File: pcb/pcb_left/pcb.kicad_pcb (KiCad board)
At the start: 2 copper layers, 154 x 108.3 mm, 62 parts, among them J1 OLED_128x32, U1 Nice_Nano_V2

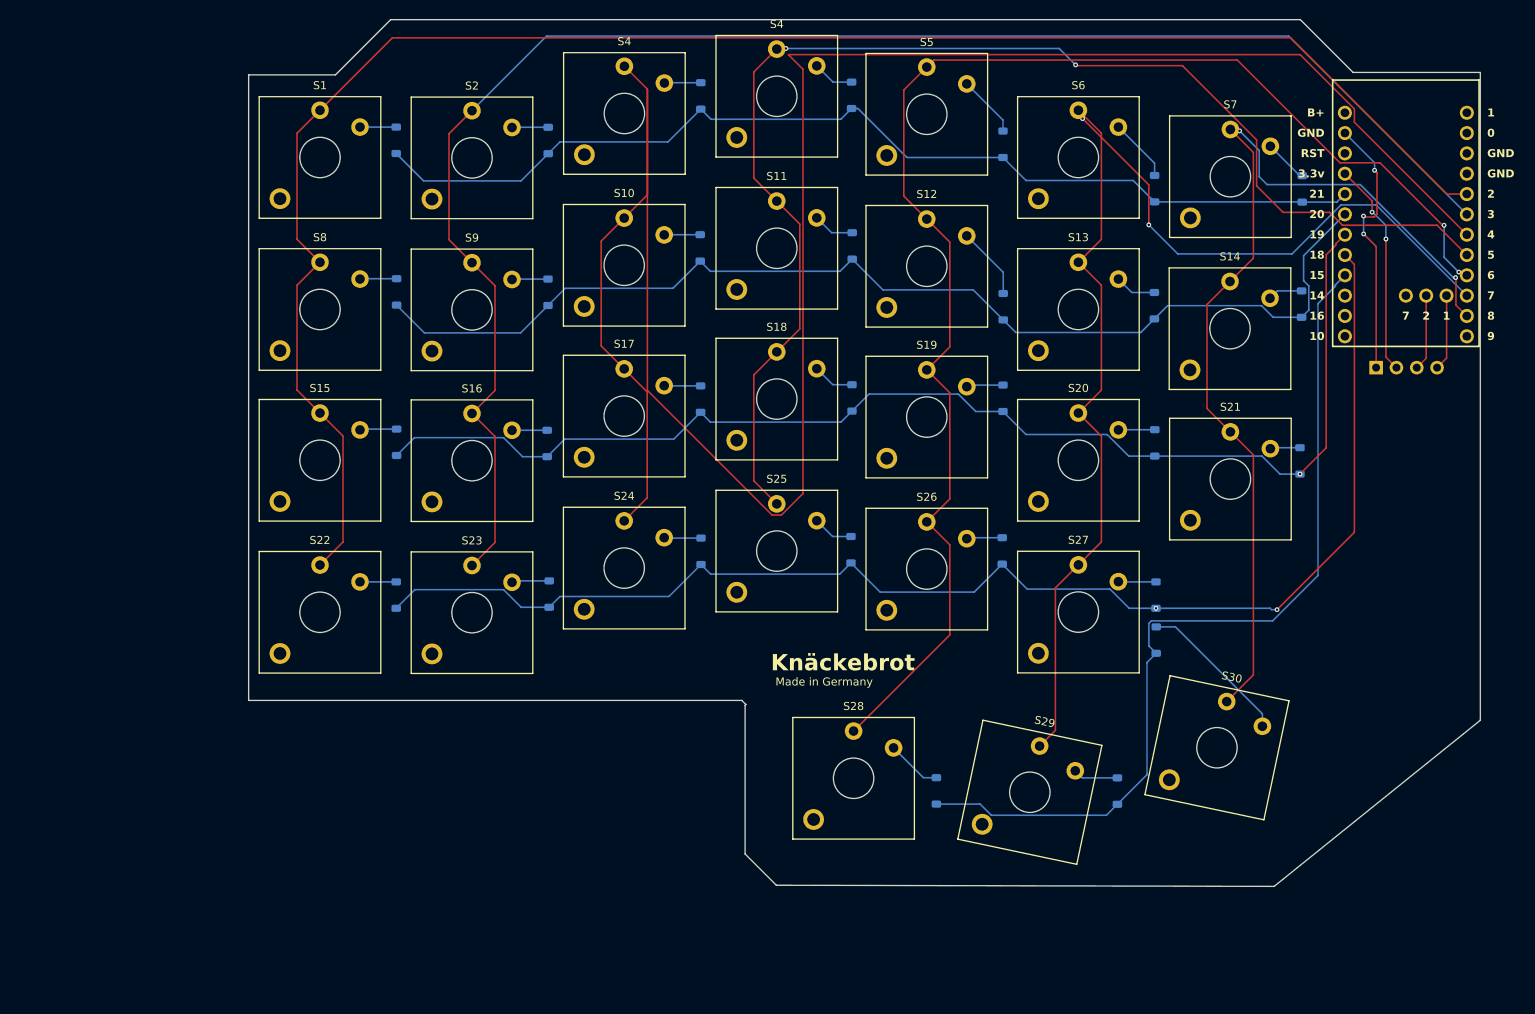
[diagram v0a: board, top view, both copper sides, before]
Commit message: Upadate v1.00
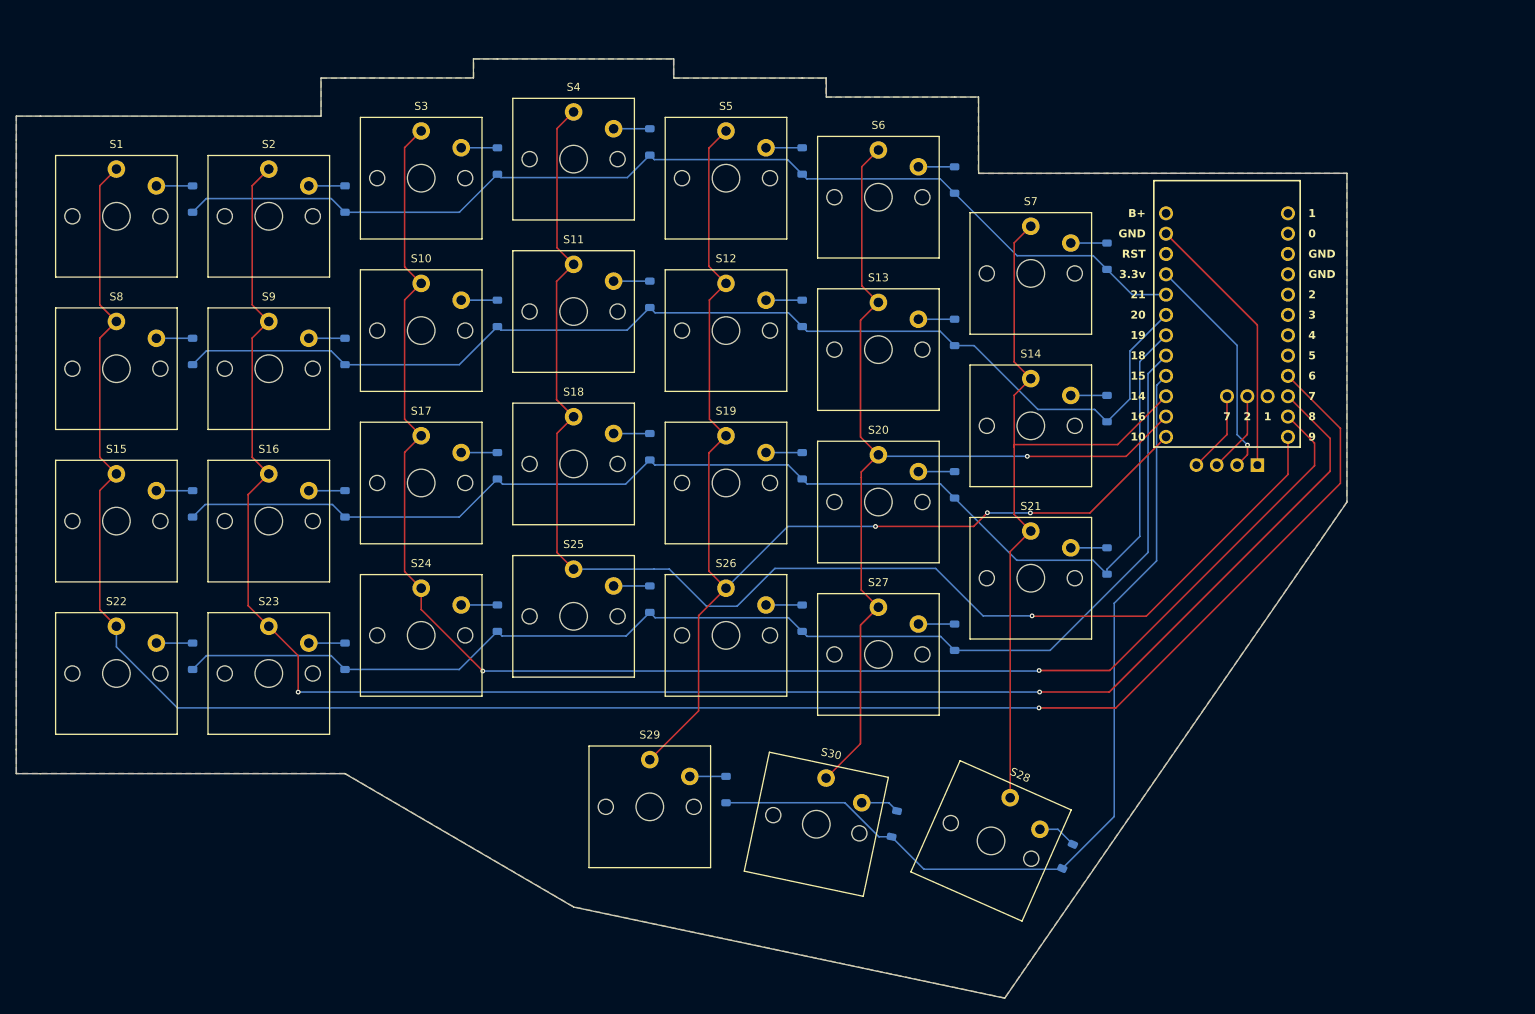
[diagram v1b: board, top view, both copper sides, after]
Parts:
- removed the S4 at (107.8, 47.8)
- removed the S4 at (126.8, 45.6)
- added S3: Keyswitch, ScottoKeebs_Choc:Choc_V1, F.Cu at (82.4, 55.9)
- added S4: Keyswitch, ScottoKeebs_Choc:Choc_V1, F.Cu at (101.4, 53.5)
- D1, D10, D11, D12, D13, D14, D15, D16, D17, D18, D19, D2, D20, D21, D22, D23, D24, D25, D26, D27, D28, D29, D3, D30, D4, D5, D6, D7, D8, D9: footprint Diode_SMD:D_SOD-123 -> ScottoKeebs_Components:Diode_SOD-123
- S1, S10, S11, S12, S13, S14, S15, S16, S17, S18, S19, S2, S20, S21, S22, S23, S24, S25, S26, S27, S28, S29, S30, S5, S6, S7, S8, S9: footprint ScottoKeebs_Choc:Choc_V2 -> ScottoKeebs_Choc:Choc_V1
- moved S30 51.0 mm to (131.8, 136.6)
- moved D29 48.9 mm to (120.5, 132.3)
- moved S29 47.5 mm to (111.0, 134.5), turned to 0 degrees
- moved D30 40.0 mm to (141.5, 136.6), turned to 78.06 degrees
- moved J1 37.7 mm to (177.1, 93.4), turned to 90 degrees
- moved S21 27.9 mm to (158.6, 105.9)
- moved S7 27.7 mm to (158.6, 67.8)
- moved S14 27.7 mm to (158.6, 86.8)
- moved D14 27.6 mm to (168.1, 84.7)
- moved D21 27.2 mm to (168.1, 103.7)
- moved D24 26.8 mm to (91.9, 110.9)
- moved D17 26.7 mm to (91.9, 91.8)
- moved S24 26.7 mm to (82.4, 113.0)
- moved S17 26.7 mm to (82.4, 94.0)
- moved D3 26.7 mm to (91.9, 53.7)
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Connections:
- net Row_0_L renamed row 0
- net Row_1_L renamed row 1
- net Row_2_L renamed row 2
- net Row_3_L renamed row 3
- net Row_4_L renamed row 4
- S1 pad 1: Col_0_L -> column 0
- S10 pad 1: Col_2_L -> column 2
- S11 pad 1: Col_3_L -> column 3
- S12 pad 1: Col_4_L -> column 4
- S13 pad 1: Col_5_L -> column 5
- S14 pad 1: Col_6_L -> column 6
- S15 pad 1: Col_0_L -> column 0
- S16 pad 1: Col_1_L -> column 1
- S17 pad 1: Col_2_L -> column 2
- S18 pad 1: Col_3_L -> column 3
- S19 pad 1: Col_4_L -> column 4
- S2 pad 1: Col_1_L -> column 1
- S20 pad 1: Col_5_L -> column 5
- S21 pad 1: Col_6_L -> column 6
- S22 pad 1: Col_0_L -> column 0
- S23 pad 1: Col_1_L -> column 1
- S24 pad 1: Col_2_L -> column 2
- S25 pad 1: Col_3_L -> column 3
- S26 pad 1: Col_4_L -> column 4
- S27 pad 1: Col_5_L -> column 5
- S28 pad 1: Col_4_L -> column 6
- S29 pad 1: Col_5_L -> column 4
- S30 pad 1: Col_6_L -> column 5
- S5 pad 1: Col_4_L -> column 4
- S6 pad 1: Col_5_L -> column 5
- S7 pad 1: Col_6_L -> column 6
- S8 pad 1: Col_0_L -> column 0
- S9 pad 1: Col_1_L -> column 1
- U1 pad 10: Col_5_L -> column 1
- U1 pad 11: Col_6_L -> column 2
- U1 pad 12: unconnected-(U1-9-Pad12) -> column 3
- U1 pad 13: unconnected-(U1-10-Pad13) -> column 4
- U1 pad 14: unconnected-(U1-16-Pad14) -> column 5
- U1 pad 15: unconnected-(U1-14-Pad15) -> column 6
- U1 pad 25: SDA -> unconnected-(U1-1-Pad25)
- U1 pad 27: unconnected-(U1-7-Pad27) -> SDA
- U1 pad 5: Col_0_L -> unconnected-(U1-2-Pad5)
- U1 pad 6: Col_1_L -> unconnected-(U1-3-Pad6)
- U1 pad 7: Col_2_L -> unconnected-(U1-4-Pad7)
- U1 pad 8: Col_3_L -> unconnected-(U1-5-Pad8)
- U1 pad 9: Col_4_L -> column 0
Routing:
- net Col_2_L: track 279.4 -> 0.00 mm
- net column 0: track 0.00 -> 248.8 mm, vias 0 -> 1
- net column 1: track 0.00 -> 224.5 mm, vias 0 -> 2
- net Col_0_L: track 219.2 -> 0.00 mm
- net Col_1_L: track 201.4 -> 0.00 mm
- net column 2: track 0.00 -> 198.0 mm, vias 0 -> 2
- net Col_4_L: track 176.5 -> 0.00 mm, vias 2 -> 0
- net column 3: track 0.00 -> 170.0 mm, vias 0 -> 1
- net Col_3_L: track 163.2 -> 0.00 mm, vias 2 -> 0
- net Col_5_L: track 153.8 -> 0.00 mm, vias 2 -> 0
- net column 4: track 0.00 -> 150.7 mm, vias 0 -> 3
- net column 5: track 0.00 -> 124.7 mm, vias 0 -> 1
- net Col_6_L: track 120.9 -> 0.00 mm, vias 2 -> 0
- net column 6: track 0.00 -> 97.8 mm
- net Net-(D30-A): track 19.3 -> 4.83 mm
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- added copper zone on B.Cu, net GND
- added copper zone on F.Cu, net GND
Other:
- board size 154 x 108.3 mm -> 166.4 x 117.4 mm
- board text removed: "Knäckebrot"
- board text removed: "Made in Germany"
